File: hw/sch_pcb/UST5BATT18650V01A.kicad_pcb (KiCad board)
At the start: 2 copper layers, 100 x 78 mm, 25 parts, among them J1 SM03B-GHS-TB, J2 SM03B-GHS-TB, X1 TPS63060

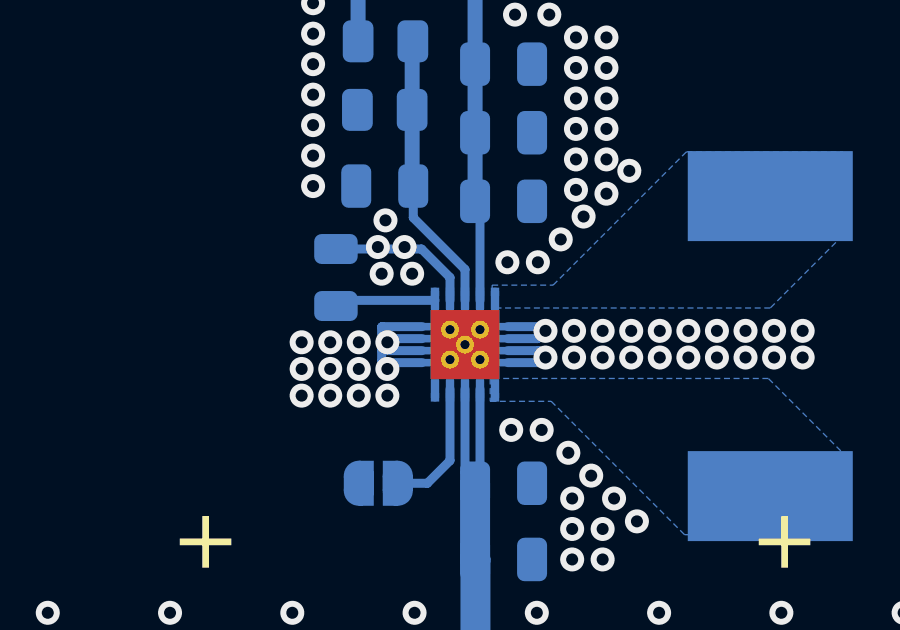
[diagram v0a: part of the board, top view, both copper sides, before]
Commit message: Edit PCB
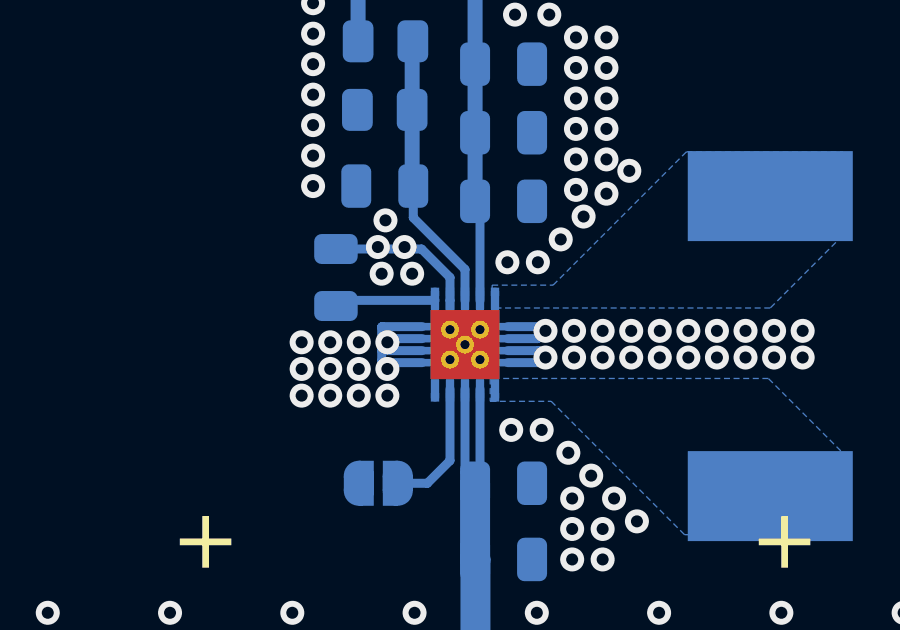
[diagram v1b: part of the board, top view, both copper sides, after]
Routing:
- net GND: track 16.9 -> 17.9 mm
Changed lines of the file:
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@@
   (segment (start 155.18 118.985) (end 155.321 119.126) (width 0.3) (layer "B.Cu") (net 1))
   (segment (start 155.062 119.385) (end 155.321 119.126) (width 0.3) (layer "B.Cu") (net 1))
+  (segment (start 152.138 118.11) (end 152.138 119.085) (width 0.3) (layer "B.Cu") (net 1))
   (segment (start 154.063 118.985) (end 155.18 118.985) (width 0.3) (layer "B.Cu") (net 1))
   (segment (start 149.86 119.38) (end 149.86 118.999) (width 0.3) (layer "B.Cu") (net 1))

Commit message: Edit UST_ID and B.FAB
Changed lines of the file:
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@@
       (effects (font (size 1 1) (thickness 0.15)) (justify mirror))
     )
-    (fp_text value "10uF" (at 0 -1.68) (layer "B.Fab")
+    (fp_text value "10uF" (at 0 -1.68) (layer "B.Fab") hide
       (effects (font (size 1 1) (thickness 0.15)) (justify mirror))
     )
@@
       (effects (font (size 1 1) (thickness 0.15)) (justify mirror))
     )
-    (fp_text value "10uF" (at 0 -1.68) (layer "B.Fab")
+    (fp_text value "10uF" (at 0 -1.68) (layer "B.Fab") hide
       (effects (font (size 1 1) (thickness 0.15)) (justify mirror))
     )
@@
       (effects (font (size 1 1) (thickness 0.15)) (justify mirror))
     )
-    (fp_text value "100k" (at 0 -1.65) (layer "B.Fab")
+    (fp_text value "100k" (at 0 -1.65) (layer "B.Fab") hide
       (effects (font (size 1 1) (thickness 0.15)) (justify mirror))
     )
@@
       (effects (font (size 1 1) (thickness 0.15)) (justify mirror))
     )
-    (fp_text value "10p" (at 0 -1.68) (layer "B.Fab")
+    (fp_text value "10p" (at 0 -1.68) (layer "B.Fab") hide
       (effects (font (size 1 1) (thickness 0.15)) (justify mirror))
     )
@@
       (effects (font (size 1 1) (thickness 0.15)) (justify mirror))
     )
-    (fp_text value "560k" (at 0 -1.65) (layer "B.Fab")
+    (fp_text value "560k" (at 0 -1.65) (layer "B.Fab") hide
       (effects (font (size 1 1) (thickness 0.15)) (justify mirror))
     )
@@
       (effects (font (size 1 1) (thickness 0.15)) (justify mirror))
     )
-    (fp_text value "47uF/6V3" (at 0 -1.68) (layer "B.Fab")
+    (fp_text value "47uF/6V3" (at 0 -1.68) (layer "B.Fab") hide
       (effects (font (size 1 1) (thickness 0.15)) (justify mirror))
     )
@@
       (effects (font (size 1 1) (thickness 0.15)) (justify mirror))
     )
-    (fp_text value "SolderJumper_2_Open" (at 0 -1.9) (layer "B.Fab")
+    (fp_text value "SolderJumper_2_Open" (at 0 -1.9) (layer "B.Fab") hide
       (effects (font (size 1 1) (thickness 0.15)) (justify mirror))
     )
@@
         (gr_circle (center 0 0.25) (end 0.5 0.25) (width 0) (fill yes))
         (gr_poly (pts
+            (xy 0.5 0.75)
+            (xy 0 0.75)
+            (xy 0 -0.75)
             (xy 0.5 -0.75)
-            (xy 0 -0.75)
-            (xy 0 0.75)
-            (xy 0.5 0.75)
           ) (width 0) (fill yes))
       ))
@@
         (gr_circle (center 0 0.25) (end 0.5 0.25) (width 0) (fill yes))
         (gr_poly (pts
+            (xy 0 0.75)
+            (xy -0.5 0.75)
+            (xy -0.5 -0.75)
             (xy 0 -0.75)
-            (xy -0.5 -0.75)
-            (xy -0.5 0.75)
-            (xy 0 0.75)
           ) (width 0) (fill yes))
       ))
@@
       (effects (font (size 1 1) (thickness 0.15)) (justify mirror))
     )
-    (fp_text value "100nF" (at 0 -1.68 -270) (layer "B.Fab")
+    (fp_text value "100nF" (at 0 -1.68 -270) (layer "B.Fab") hide
       (effects (font (size 1 1) (thickness 0.15)) (justify mirror))
     )
@@
       (effects (font (size 1 1) (thickness 0.15)) (justify mirror))
     )
-    (fp_text value "47uF/6V3" (at 0 -1.68) (layer "B.Fab")
+    (fp_text value "47uF/6V3" (at 0 -1.68) (layer "B.Fab") hide
       (effects (font (size 1 1) (thickness 0.15)) (justify mirror))
     )
@@
       (effects (font (size 1 1) (thickness 0.15)) (justify mirror))
     )
-    (fp_text value "47uF/6V3" (at 0 -1.68) (layer "B.Fab")
+    (fp_text value "47uF/6V3" (at 0 -1.68) (layer "B.Fab") hide
       (effects (font (size 1 1) (thickness 0.15)) (justify mirror))
     )
@@
       (effects (font (size 1 1) (thickness 0.15)) (justify mirror))
     )
-    (fp_text value "20k" (at 0 -1.65) (layer "B.Fab")
+    (fp_text value "20k" (at 0 -1.65) (layer "B.Fab") hide
       (effects (font (size 1 1) (thickness 0.15)) (justify mirror))
     )
@@
       (effects (font (size 1 1) (thickness 0.15)) (justify mirror))
     )
-    (fp_text value "TPS63060" (at 0 -2.8 90) (layer "B.Fab")
-      (effects (font (size 1 1) (thickness 0.15)) (justify mirror))
-    )
+    (fp_text value "TPS63060" (at 0 -2.8 90) (layer "B.Fab") hide
+      (effects (font (size 1 1) (thickness 0.15)) (justify mirror))
+    )
